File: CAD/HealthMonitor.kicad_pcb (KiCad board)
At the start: 2 copper layers, 58.7 x 33.3 mm, 114 parts, among them J1 BAT_T, J10 SDA, J11 SCL, J12 DIS_SW, J13 BAT_CHRG, J14 USBDP, J15 USBDM, J16 USB_V, J17 VBUS, J18 D+, J19 D-, J2 TEG+, J20 SDA, J21 SCL, J22 VCC, J23 GND, J24 BAT_CHRG, J25 DIS_SW, J3 TEG-, J4 BAT-, J5 BAT+, J6 USB_C_Receptacle_USB2.0, J7 Conn_02x05_Odd_Even, J8 VCC, J9 GND, U1 MAX17048G+T10, U10 AT24CS02-XHM, U11 BT832L, U12 CP2102N-A01-GQFN24, U13 ADG884BRMZ, U2 ADP5092ACPZ-1-R7, U3 LTC4079IDD-PBF, U4 LD39015M33R, U5 BH1792GLC, U6 LSM6DS33TR, U7 TXB0104RUT, U8 MAX1921EUT18+, U9 MAX86141ENP+, Y1 ABS06-32.768KHZ-T

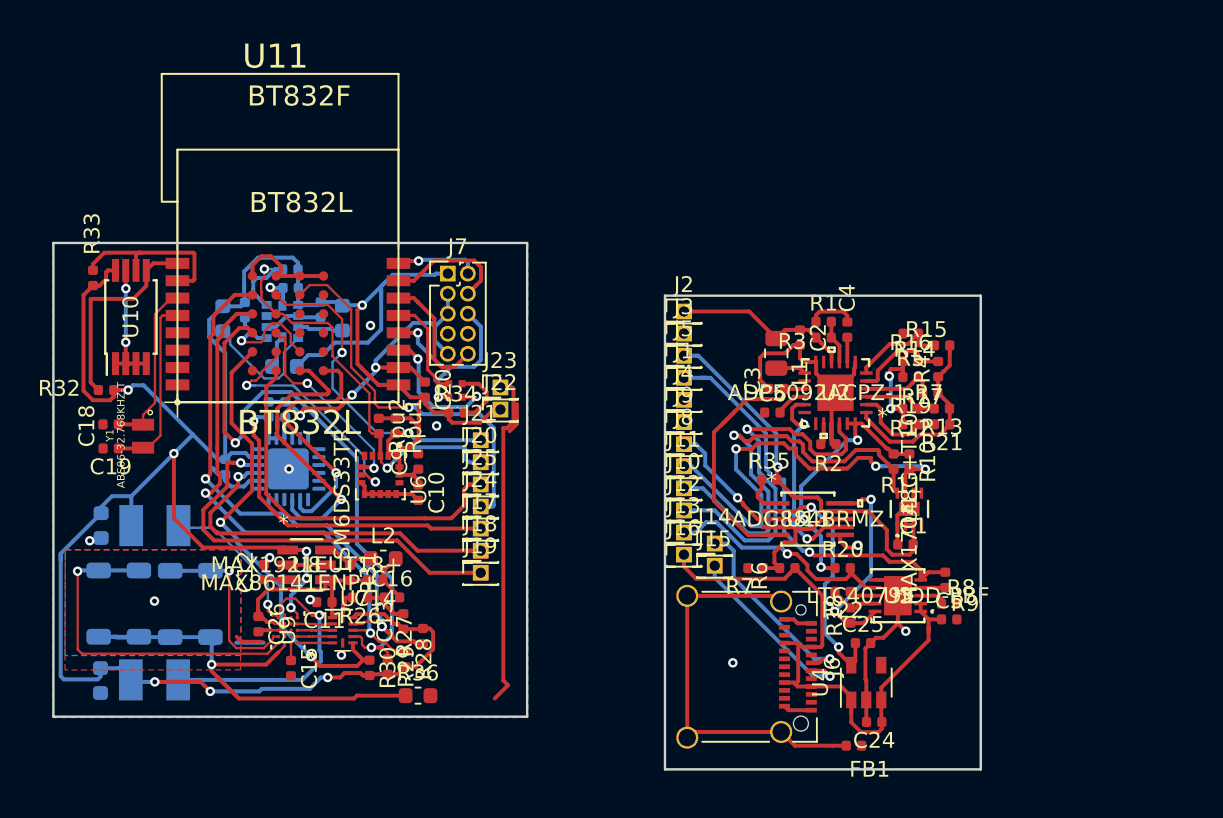
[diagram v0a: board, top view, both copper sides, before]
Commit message: Generated gerbers
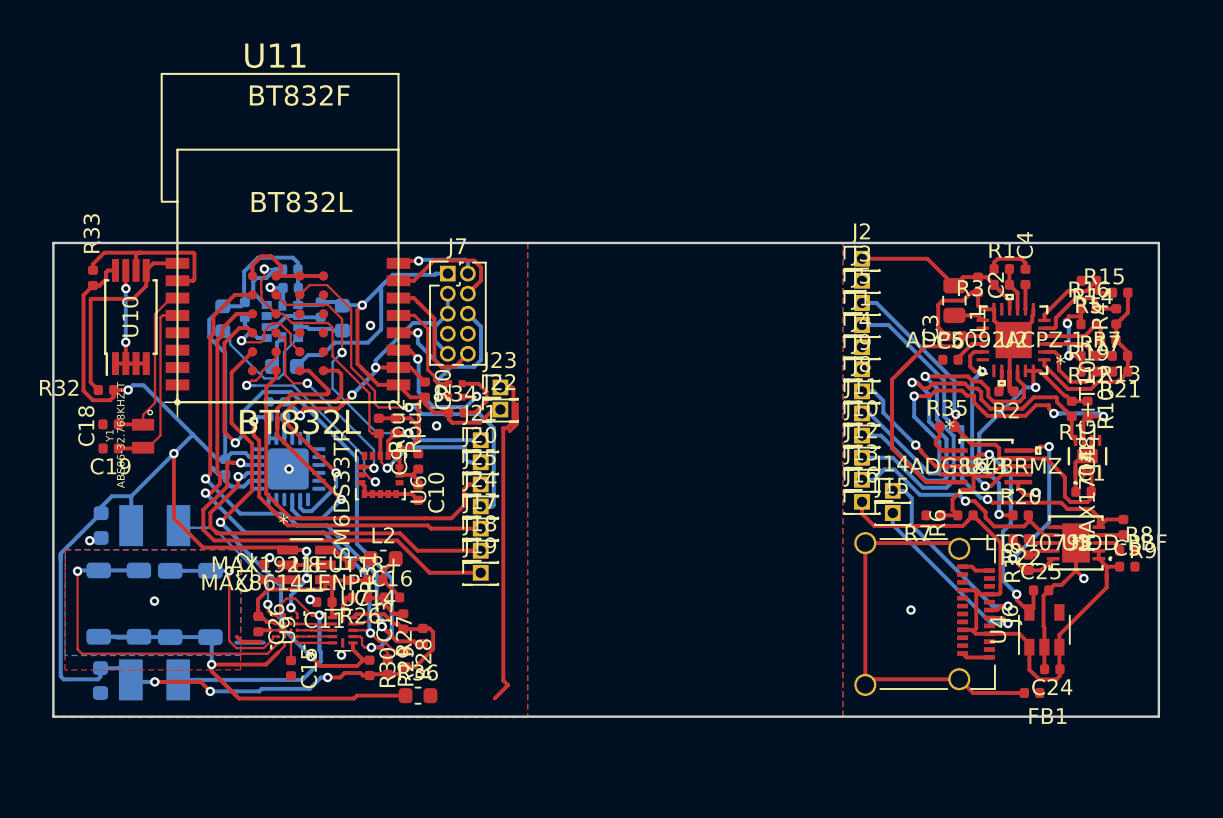
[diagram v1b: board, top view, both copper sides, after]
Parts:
- J6: footprint Connector_USB:USB_C_Receptacle_Amphenol_12401610E4-2A_CircularHoles -> footprints:USB_C_Receptacle_Amphenol_12401610E4-2A_CircularHoles
- moved C24 11.8 mm to (165.2, 123.1)
- moved C25 11.8 mm to (164.5, 118.1)
- moved C5 11.8 mm to (170.0, 116.6)
- moved FB1 11.8 mm to (163.9, 124.6)
- moved J1 11.8 mm to (153.2, 101.3)
- moved J10 11.8 mm to (153.2, 108.3)
- moved J11 11.8 mm to (153.2, 106.9)
- moved J12 11.8 mm to (153.2, 109.7)
- moved J13 11.8 mm to (153.2, 111.1)
- moved J14 11.8 mm to (155.1, 111.8)
- moved J15 11.8 mm to (155.1, 113.2)
- moved J2 11.8 mm to (153.2, 97.1)
- moved J4 11.8 mm to (153.2, 102.7)
- moved J5 11.8 mm to (153.2, 99.9)
- moved J6 11.8 mm to (156.2, 119.6)
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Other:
- board size 58.7 x 33.3 mm -> 70 x 30 mm

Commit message: Updated PCB and generated gerbers
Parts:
- C12, C16: value 4.7µF -> 4.7u
- C14: value 5600pF -> 5600p
- C15: value 10µF 10V -> 10u
- C26: value 1µf 10V -> 1u
- L2: value 4.7µH -> 4.7u
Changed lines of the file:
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@@
     (0 F.Cu signal)
     (31 B.Cu signal)
-    (32 B.Adhes user)
-    (33 F.Adhes user)
+    (32 B.Adhes user hide)
+    (33 F.Adhes user hide)
     (34 B.Paste user)
     (35 F.Paste user)
-    (36 B.SilkS user)
-    (37 F.SilkS user)
+    (36 B.SilkS user hide)
+    (37 F.SilkS user hide)
     (38 B.Mask user)
     (39 F.Mask user)
@@
     (41 Cmts.User user)
     (42 Eco1.User user)
-    (43 Eco2.User user)
-    (44 Edge.Cuts user)
+    (43 Eco2.User user hide)
+    (44 Edge.Cuts user hide)
     (45 Margin user)
     (46 B.CrtYd user)
     (47 F.CrtYd user)
-    (48 B.Fab user hide)
-    (49 F.Fab user hide)
+    (48 B.Fab user)
+    (49 F.Fab user)
   )
   (setup
@@
     (pad_to_mask_clearance 0.051)
     (solder_mask_min_width 0.25)
+    (pad_to_paste_clearance -0.1)
     (aux_axis_origin 0 0)
     (visible_elements FFFFFF7F)
@@
       (effects (font (size 1 1) (thickness 0.15)))
     )
-    (fp_text value "1µf 10V" (at 0 1.17 270) (layer F.Fab)
+    (fp_text value 1u (at 0 1.17 270) (layer F.Fab)
       (effects (font (size 1 1) (thickness 0.15)))
     )
@@
       (effects (font (size 1 1) (thickness 0.15)))
     )
-    (fp_text value 4.7µF (at 0 1.17 90) (layer F.Fab)
+    (fp_text value 4.7u (at 0 1.17 90) (layer F.Fab)
       (effects (font (size 1 1) (thickness 0.15)))
     )
@@
       (effects (font (size 1 1) (thickness 0.15)))
     )
-    (fp_text value 5600pF (at 0 1.17 180) (layer F.Fab)
+    (fp_text value 5600p (at 0 1.17 180) (layer F.Fab)
       (effects (font (size 1 1) (thickness 0.15)))
     )
@@
       (effects (font (size 1 1) (thickness 0.15)))
     )
-    (fp_text value "10µF 10V" (at 0 1.17 270) (layer F.Fab)
+    (fp_text value 10u (at 0 1.17 270) (layer F.Fab)
       (effects (font (size 1 1) (thickness 0.15)))
     )
@@
       (effects (font (size 1 1) (thickness 0.15)))
     )
-    (fp_text value 4.7µF (at 0 1.17) (layer F.Fab)
+    (fp_text value 4.7u (at 0 1.17) (layer F.Fab)
       (effects (font (size 1 1) (thickness 0.15)))
     )
@@
       (effects (font (size 1 1) (thickness 0.15)))
     )
-    (fp_text value 4.7µH (at 0 1.43) (layer F.Fab)
+    (fp_text value 4.7u (at 0 1.43) (layer F.Fab)
       (effects (font (size 1 1) (thickness 0.15)))
     )
@@
   (segment (start 166.65 103.26) (end 166.28 103.26) (width 0.25) (layer F.Cu) (net 3))
   (segment (start 166.28 103.26) (end 166.65 103.26) (width 0.25) (layer F.Cu) (net 3))
-  (via (at 166.28 103.26) (size 0.6) (drill 0.3) (layers F.Cu B.Cu) (net 3) (status 1000000))
+  (via (at 166.28 103.26) (size 0.6) (drill 0.3) (layers F.Cu B.Cu) (net 3))
   (segment (start 161.53 100.309999) (end 161.53 100.245) (width 0.25) (layer F.Cu) (net 3))
   (segment (start 161.53 100.309999) (end 160.766408 100.309999) (width 0.25) (layer F.Cu) (net 3))
@@
     (connect_pads (clearance 0.2))
     (min_thickness 0.2)
-    (fill yes (arc_segments 16) (thermal_gap 0.4) (thermal_bridge_width 0.4))
+    (fill (arc_segments 16) (thermal_gap 0.4) (thermal_bridge_width 0.4))
     (polygon
       (pts
@@
     (connect_pads (clearance 0.254))
     (min_thickness 0.254)
-    (fill yes (arc_segments 16) (thermal_gap 0.508) (thermal_bridge_width 0.508))
+    (fill (arc_segments 16) (thermal_gap 0.508) (thermal_bridge_width 0.508))
     (polygon
       (pts
@@
     (connect_pads (clearance 0.2))
     (min_thickness 0.2)
-    (fill yes (arc_segments 16) (thermal_gap 0.4) (thermal_bridge_width 0.4))
+    (fill (arc_segments 16) (thermal_gap 0.4) (thermal_bridge_width 0.4))
     (polygon
       (pts
@@
     (connect_pads (clearance 0.2))
     (min_thickness 0.2)
-    (fill yes (arc_segments 16) (thermal_gap 0.4) (thermal_bridge_width 0.4))
+    (fill (arc_segments 16) (thermal_gap 0.4) (thermal_bridge_width 0.4))
     (polygon
       (pts
@@
     (connect_pads (clearance 0.2))
     (min_thickness 0.2)
-    (fill yes (arc_segments 16) (thermal_gap 0.4) (thermal_bridge_width 0.4))
+    (fill (arc_segments 16) (thermal_gap 0.4) (thermal_bridge_width 0.4))
     (polygon
       (pts
@@
     (connect_pads (clearance 0.2))
     (min_thickness 0.2)
-    (fill yes (arc_segments 16) (thermal_gap 0.4) (thermal_bridge_width 0.4))
+    (fill (arc_segments 16) (thermal_gap 0.4) (thermal_bridge_width 0.4))
     (polygon
       (pts
